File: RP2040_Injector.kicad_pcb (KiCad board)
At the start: 2 copper layers, 49.8 x 14 mm, 36 parts, among them J1 USB-A, J2 Conn_01x02, U1 NCP1117-3.3_SOT223, U2 W25Q128JVS, U3 RP2040

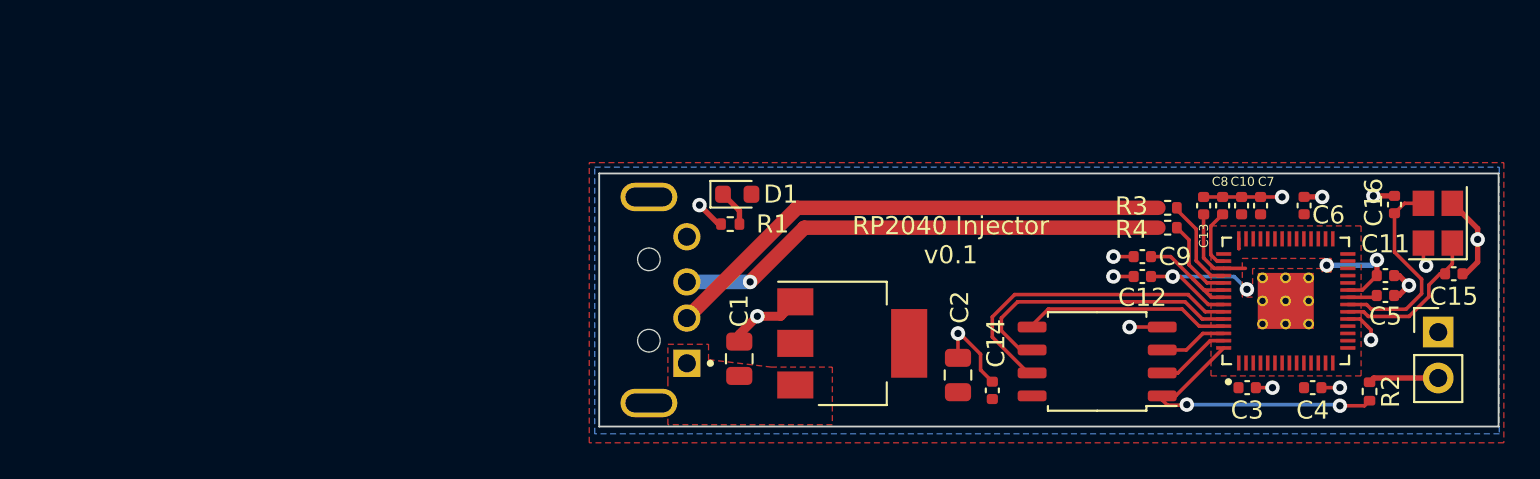
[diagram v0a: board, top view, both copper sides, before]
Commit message: Started v0.2
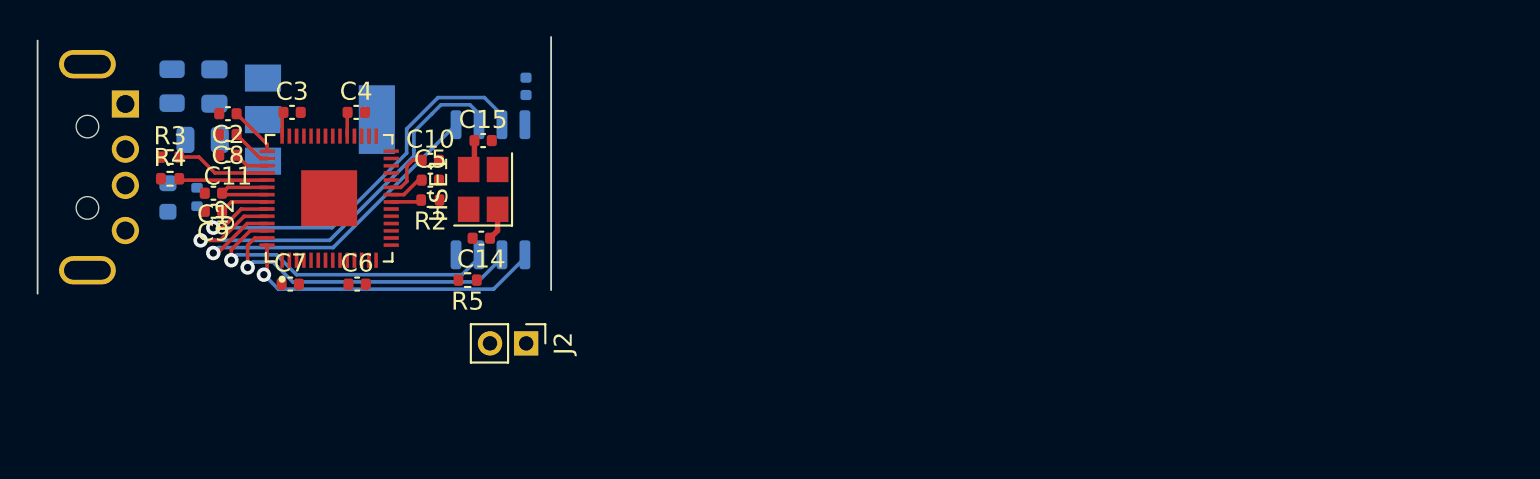
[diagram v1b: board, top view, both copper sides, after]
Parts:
- removed ? (x9): , 
- added F1: 0805L050WR, Fuse:Fuse_0805_2012Metric, B.Cu at (100.9, 89.3)
- added R5: 1k, Resistor_SMD:R_0402_1005Metric, F.Cu at (117.3, 100.0)
- C1, C2: value 10u -> 100n; footprint Capacitor_SMD:C_0805_2012Metric -> Capacitor_SMD:C_0402_1005Metric
- C10: value 1u -> 100n
- C11, C8: value 100n -> 1u
- C12: value 100n -> 10u; footprint Capacitor_SMD:C_0402_1005Metric -> Capacitor_SMD:C_0805_2012Metric; moved to B.Cu
- C13: value 1u -> 10u; footprint Capacitor_SMD:C_0402_1005Metric -> Capacitor_SMD:C_0805_2012Metric; moved to B.Cu
- C14: value 100n -> 20p
- C15: value 15p -> 20p
- C16: value 15p -> 100n; moved to B.Cu
- D1, J1, R1, U1: moved to B.Cu
- J2: footprint Connector_PinHeader_2.54mm:PinHeader_1x02_P2.54mm_Vertical -> Connector_PinHeader_2.00mm:PinHeader_1x02_P2.00mm_Vertical
- U2: value W25Q128JVS -> RP2040; footprint Package_SO:SOIC-8_5.23x5.23mm_P1.27mm -> RP2040:QFN40P700X700X90-57N
- U3: value RP2040 -> W25Q128JVS; footprint RP2040:QFN40P700X700X90-57N -> Package_SO:SOIC-8_5.23x5.23mm_P1.27mm; moved to B.Cu
- moved C11 64.4 mm to (104.0, 93.1), turned to 180 degrees
- moved C13 55.5 mm to (102.6, 92.2), turned to 180 degrees
- moved R3 55.3 mm to (100.8, 93.2)
- moved R4 55.3 mm to (100.8, 94.4)
- moved C8 55.2 mm to (104.0, 91.9), turned to 180 degrees
- moved C4 55.1 mm to (111.1, 90.7)
- moved C3 55.0 mm to (107.6, 90.7)
- moved C15 54.2 mm to (118.1, 92.3)
- moved C7 53.9 mm to (107.5, 100.2), turned to 0 degrees
- moved C5 53.2 mm to (115.2, 94.5)
- moved R2 53.0 mm to (115.2, 95.6), turned to 180 degrees
- moved HSE1 52.9 mm to (118.1, 95.0)
- moved C6 52.6 mm to (111.2, 100.2), turned to 0 degrees
- moved C12 52.4 mm to (103.3, 89.3), turned to -90 degrees
- moved C9 51.5 mm to (103.2, 96.2)
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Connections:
- net USB_DM renamed USB_D-
- net USB_DP renamed USB_D+
- C1 pad 1: VCC -> +3V3
- C10 pad 1: +3V3 -> +1V1
- C12 pad 1: +1V1 -> Net-(C12-Pad1)
- C13 pad 1: +1V1 -> +3V3
- C14 pad 1: +3V3 -> XIN
- C15 pad 1: XIN -> Net-(C15-Pad1)
- C16 pad 1: XOUT -> +3V3
- C9 pad 1: +3V3 -> +1V1
- HSE1 pad 3: XOUT -> Net-(C15-Pad1)
- R2 pad 1: /~{USB_BOOT} -> Net-(C15-Pad1)
- R2 pad 2: /QSPI_CSN -> XOUT
- U1 pad 3: VCC -> Net-(C12-Pad1)
- U2 pad 1: /QSPI_CSN -> +3V3
- U2 pad 2: /QSPI_SD1 -> unconnected-(U2-Pad2)
- U2 pad 3: /QSPI_SD2 -> unconnected-(U2-Pad3)
- U2 pad 4: GND -> unconnected-(U2-Pad4)
- U2 pad 5: /QSPI_SD0 -> unconnected-(U2-Pad5)
- U2 pad 6: /QSPI_SCLK -> unconnected-(U2-Pad6)
- U2 pad 7: /QSPI_SD3 -> unconnected-(U2-Pad7)
- U2 pad 8: +3V3 -> unconnected-(U2-Pad8)
- U3 pad 1: +3V3 -> /QSPI_CSN
- U3 pad 2: unconnected-(U3-Pad2) -> /QSPI_SD1
- U3 pad 3: unconnected-(U3-Pad3) -> /QSPI_SD2
- U3 pad 4: unconnected-(U3-Pad4) -> GND
- U3 pad 5: unconnected-(U3-Pad5) -> /QSPI_SD0
- U3 pad 6: unconnected-(U3-Pad6) -> /QSPI_SCLK
- U3 pad 7: unconnected-(U3-Pad7) -> /QSPI_SD3
- U3 pad 8: unconnected-(U3-Pad8) -> +3V3
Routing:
- net GND: track 33.7 -> 0.00 mm, vias 15 -> 0
- net USB_D-: track 28.6 -> 0.00 mm
- net USB_D+: track 27.3 -> 0.00 mm, vias 1 -> 0
- net /QSPI_SD2: track 3.78 -> 18.1 mm, vias 0 -> 1
- net /QSPI_SD1: track 4.14 -> 17.8 mm, vias 0 -> 1
- net +1V1: track 19.9 -> 7.43 mm, vias 4 -> 0
- net XOUT: track 11.4 -> 1.70 mm
- net /QSPI_SD0: track 11.5 -> 20.2 mm, vias 0 -> 1
- net /QSPI_SCLK: track 15.9 -> 24.3 mm, vias 0 -> 1
- net XIN: track 8.71 -> 1.77 mm
- net /QSPI_SD3: track 17.8 -> 24.1 mm, vias 0 -> 1
- net /~{USB_BOOT}: track 3.90 -> 0.00 mm
- net +3V3: track 12.5 -> 14.8 mm
- net Net-(D1-Pad1): track 2.03 -> 0.00 mm
- net Net-(C15-Pad1): track 0.00 -> 2.02 mm
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- removed copper zone on F.Cu, net +1V1
- removed copper zone on F.Cu, net +3V3
- removed copper zone on B.Cu, net GND
- removed copper zone on F.Cu, net VCC
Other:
- board size 49.8 x 14 mm -> 28.4 x 14.2 mm
- copper layers 2 -> 4
- board text removed: "BSC 8/22"
- board text removed: "RP2040 Injector v0.1"

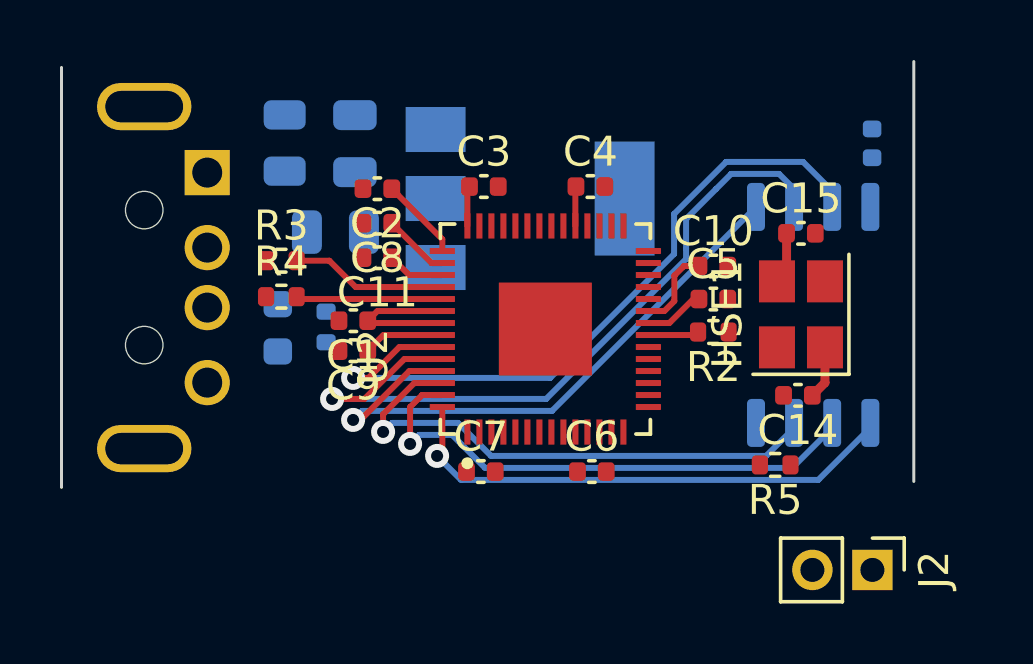
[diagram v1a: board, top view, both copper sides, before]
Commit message: Finished wiring
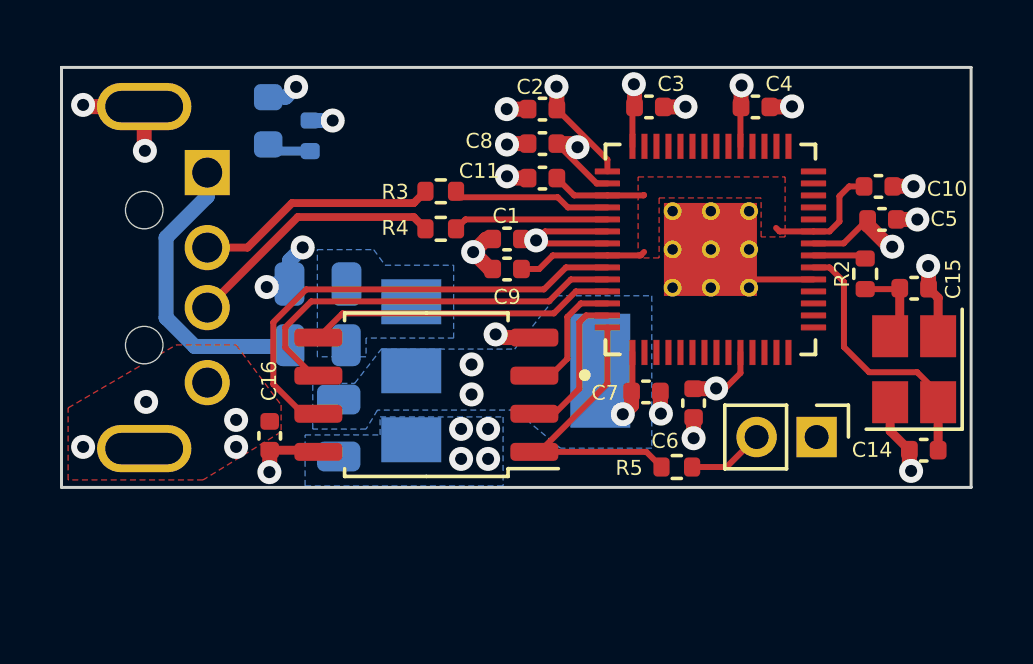
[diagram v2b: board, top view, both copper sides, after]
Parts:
- added ?: , , F.Cu at (116.4, 91.5)
- added ?: , , F.Cu at (116.4, 94.1)
- added ?: , , F.Cu at (113.8, 94.1)
- added ?: , , F.Cu at (115.1, 91.5)
- added ?: , , F.Cu at (116.4, 92.8)
- added ?: , , F.Cu at (113.8, 92.8)
- added ?: , , F.Cu at (115.1, 94.1)
- added ?: , , F.Cu at (115.1, 92.8)
- added ?: , , F.Cu at (113.8, 91.5)
- C16, U3: moved to F.Cu
- moved C16 22.3 mm to (100.4, 99.0)
- moved U3 13.2 mm to (105.6, 97.7), turned to 180 degrees
- moved D1 6.91 mm to (100.4, 88.5)
- moved F1 6.83 mm to (102.0, 96.0), turned to 0 degrees
- moved C13 6.53 mm to (102.7, 98.8), turned to -90 degrees
- moved R1 6.39 mm to (101.8, 89.0)
- moved C5 6.22 mm to (120.8, 91.8)
- moved C10 6.11 mm to (120.7, 90.7)
- moved C7 6.11 mm to (113.0, 97.6)
- moved C11 6.11 mm to (109.5, 90.4)
- moved C2 6.11 mm to (109.5, 88.1)
- moved C3 6.11 mm to (113.1, 88.1)
- moved C4 6.11 mm to (116.6, 88.1)
- moved U2 6.11 mm to (115.1, 92.8)
- moved C8 6.11 mm to (109.5, 89.3)
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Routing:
- net GND: track 0.00 -> 25.0 mm, vias 0 -> 26
- net /QSPI_SD2: track 18.1 -> 4.25 mm, vias 1 -> 0
- net +3V3: track 14.8 -> 27.7 mm, vias 0 -> 12
- net /QSPI_SD1: track 17.8 -> 5.09 mm, vias 1 -> 0
- net /QSPI_SCLK: track 24.3 -> 13.6 mm, vias 1 -> 0
- net VCC: track 0.00 -> 9.95 mm
- net /QSPI_SD0: track 20.2 -> 10.3 mm, vias 1 -> 0
- net USB_D+: track 0.00 -> 8.69 mm
- net /QSPI_SD3: track 24.1 -> 15.9 mm, vias 1 -> 0
- net USB_D-: track 0.00 -> 8.05 mm
- net /QSPI_CSN: track 17.5 -> 9.70 mm, vias 1 -> 0
- net XIN: track 1.77 -> 9.06 mm
- net +1V1: track 7.43 -> 11.6 mm
- net /~{USB_BOOT}: track 0.00 -> 2.56 mm
- net Net-(D1-Pad1): track 0.00 -> 1.49 mm
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- added copper zone on F.Cu, net +1V1
- added copper zone on B.Cu, net +3V3
- added copper zone on In2.Cu, net +3V3
- added copper zone on B.Cu, net GND
- added copper zone on F.Cu, net GND
- added copper zone on In1.Cu, net GND
- added copper zone on B.Cu, net Net-(C12-Pad1)
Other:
- board size 28.4 x 14.2 mm -> 30.3 x 14 mm

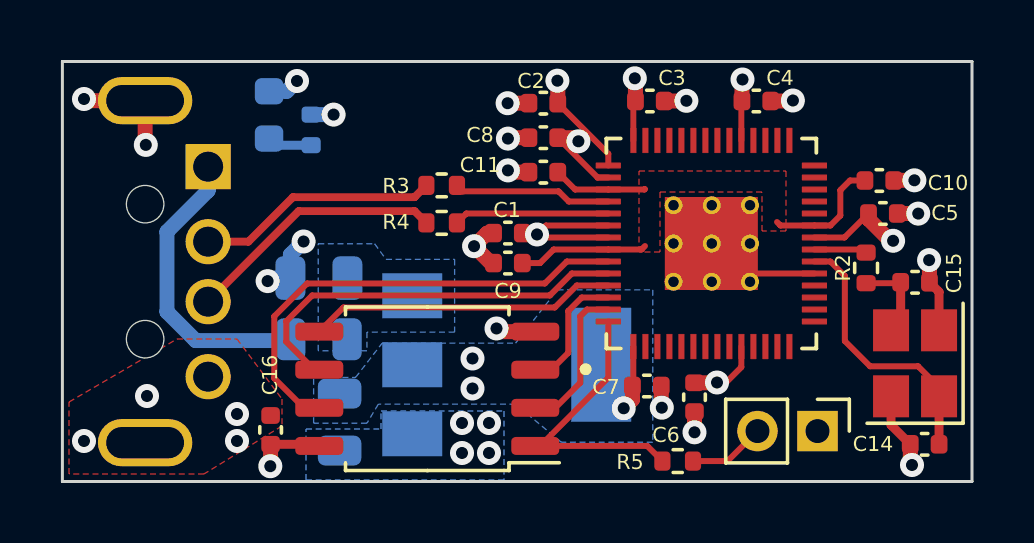
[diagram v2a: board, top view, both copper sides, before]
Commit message: Completed v0.2
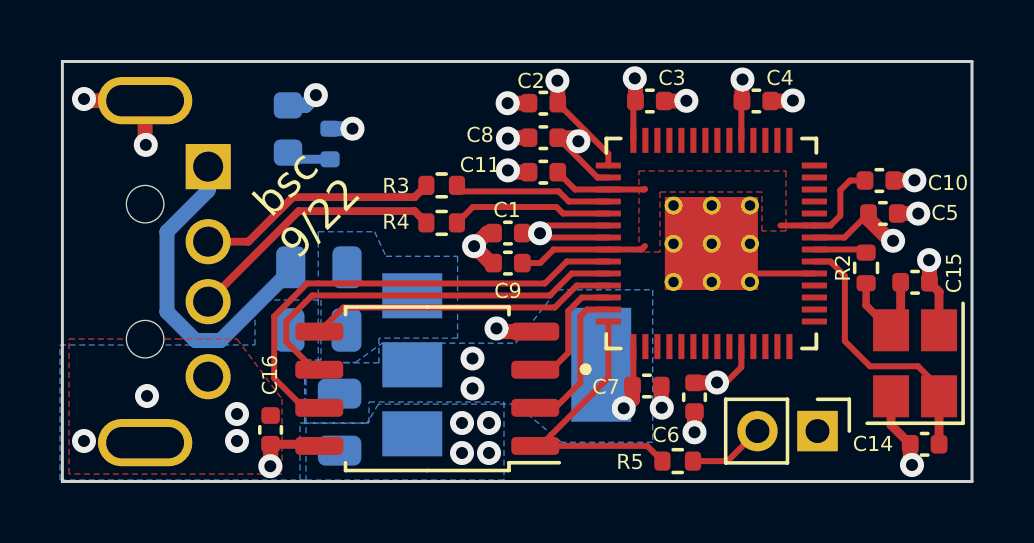
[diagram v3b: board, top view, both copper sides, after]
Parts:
- removed the ? at (116.4, 91.5)
- removed the ? at (116.4, 94.1)
- removed the ? at (113.8, 94.1)
- removed the ? at (115.1, 91.5)
- removed the ? at (116.4, 92.8)
- removed the ? at (113.8, 92.8)
- removed the ? at (115.1, 94.1)
- removed the ? at (115.1, 92.8)
- removed the ? at (113.8, 91.5)
- added ?: , , F.Cu at (116.4, 91.5)
- added ?: , , F.Cu at (115.1, 91.5)
- added ?: , , F.Cu at (115.1, 92.8)
- added ?: , , F.Cu at (113.8, 94.1)
- added ?: , , F.Cu at (116.4, 92.8)
- added ?: , , F.Cu at (116.4, 94.1)
- added ?: , , F.Cu at (113.8, 92.8)
- added ?: , , F.Cu at (113.8, 91.5)
- added ?: , , F.Cu at (115.1, 94.1)
- moved F1 2.40 mm to (102.0, 93.6)
- moved C12 1.73 mm to (102.0, 95.7)
- moved R1 0.79 mm to (102.4, 89.5)
- moved D1 0.79 mm to (101.0, 89.0)
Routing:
- net GND: track 25.0 -> 22.8 mm, vias 26 -> 24
- net VCC: track 9.95 -> 11.0 mm
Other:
- board text added: "RP2040 Injector v0.2"
- board text added: "bsc 9/22"
